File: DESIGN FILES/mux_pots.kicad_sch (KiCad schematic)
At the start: 19 parts, among them U701 CD74HC4067

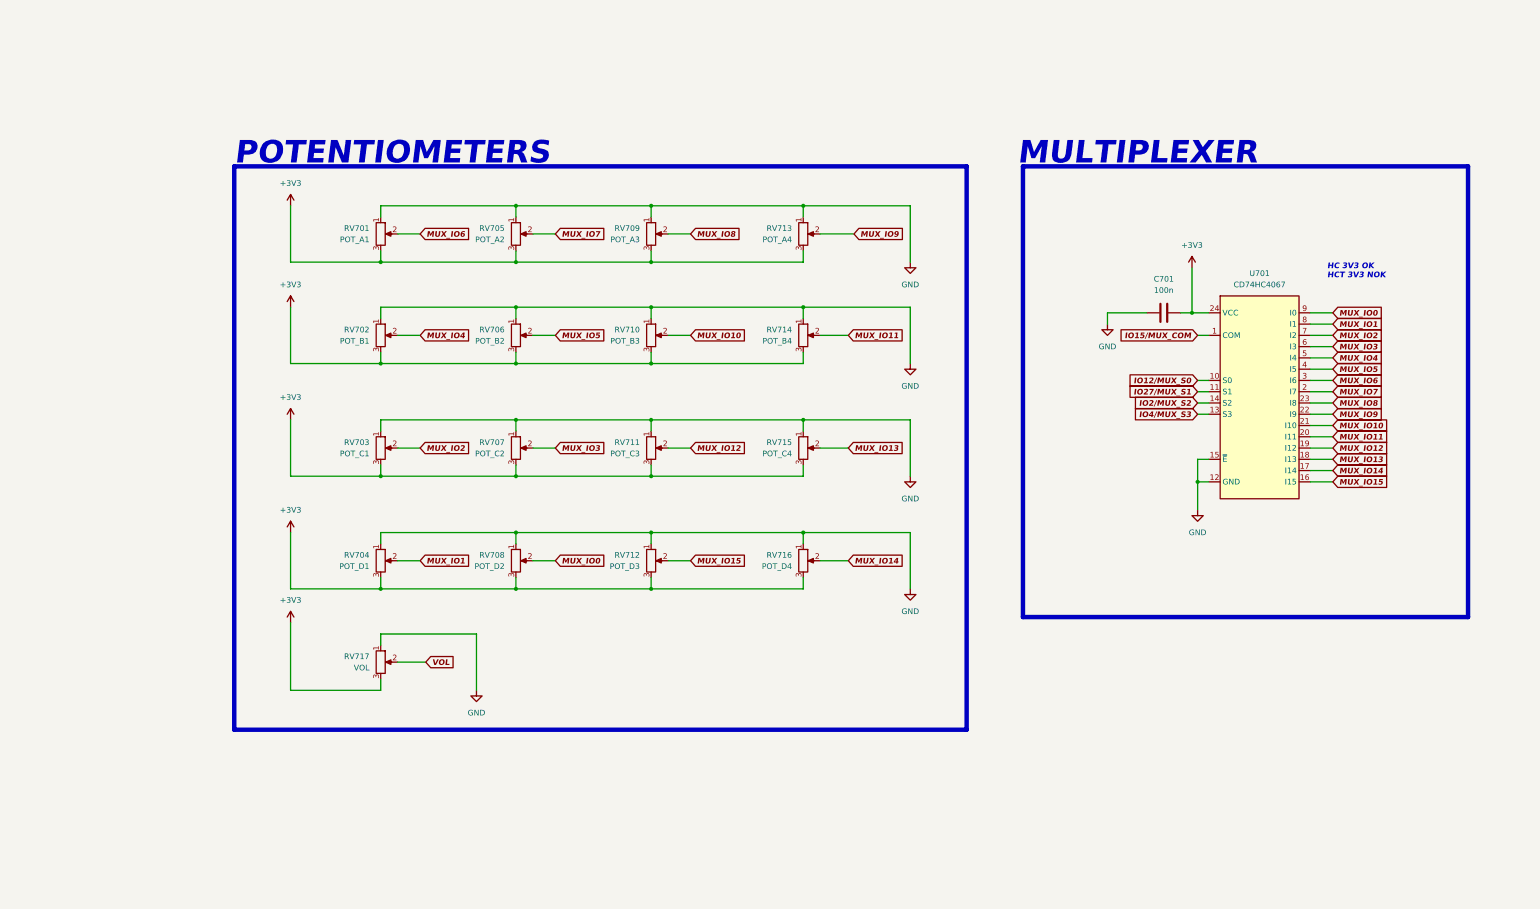
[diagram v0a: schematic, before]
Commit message: updates
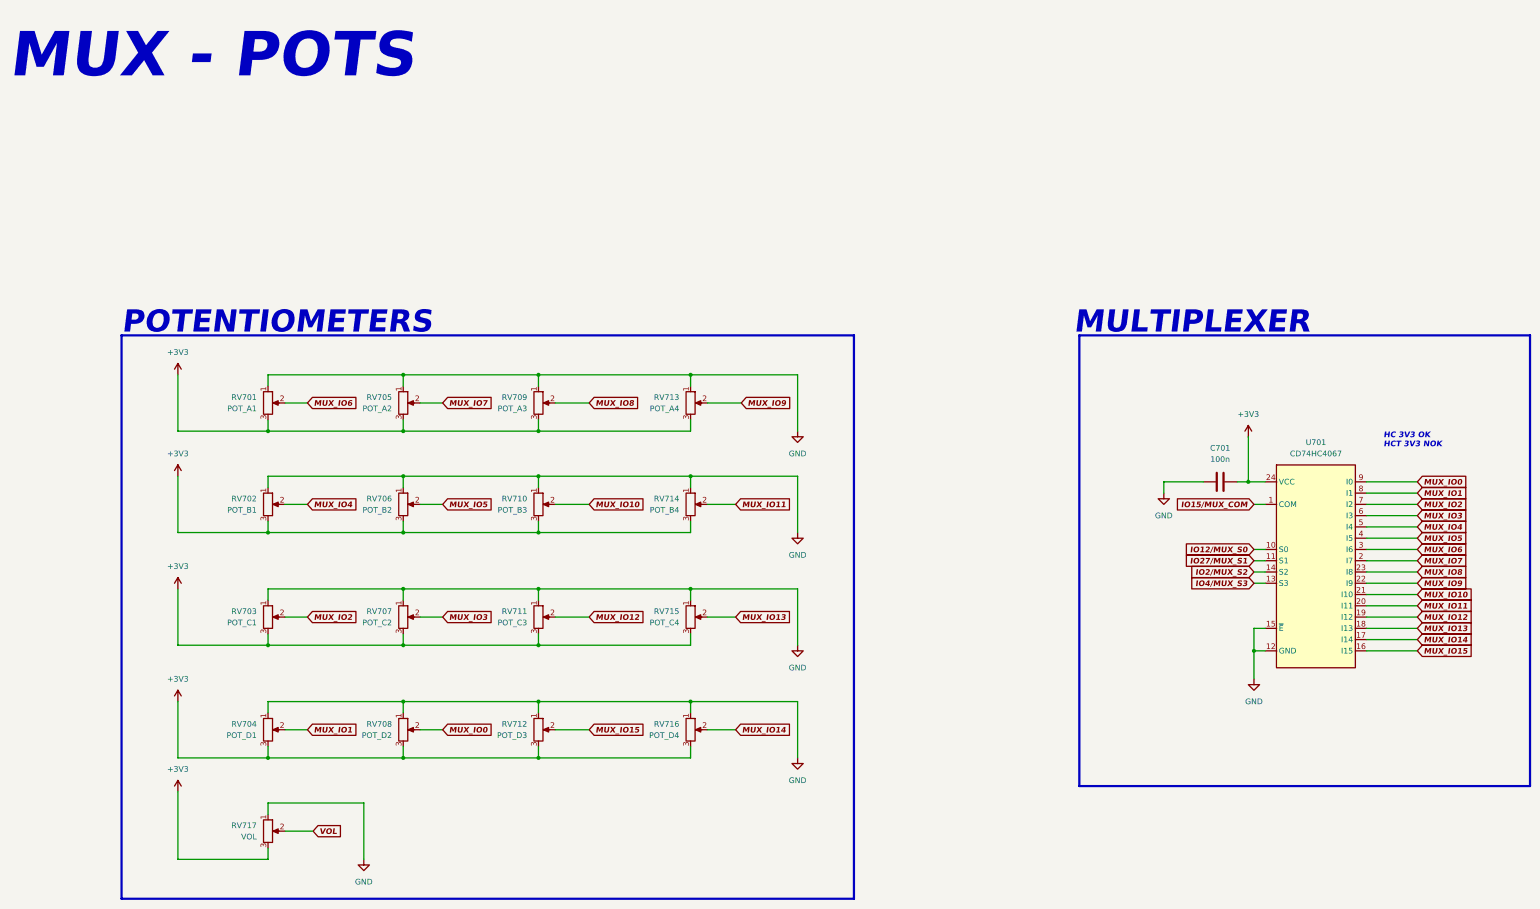
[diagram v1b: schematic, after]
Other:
- note added: "MUX - POTS"
- company: (none) -> Joël Ucedo
- title: (none) -> ESP32 SYNTH
- moved on the sheet: C701, RV701, RV702, RV703, RV704, RV705, RV706, RV707, RV708, RV709, RV710, RV711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
